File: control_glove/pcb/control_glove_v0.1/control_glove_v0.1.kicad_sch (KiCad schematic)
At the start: 14 parts, among them P1 Power_Pins, SW1 SW_Push, SW2 SW_Push, U1 UART-RF433

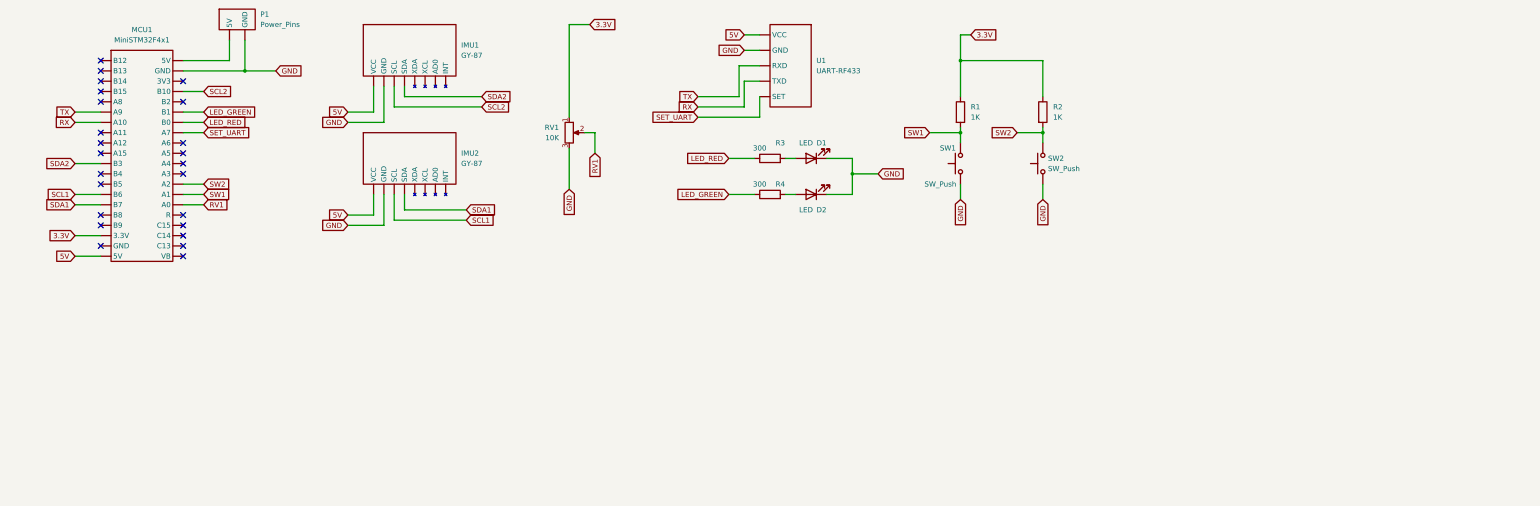
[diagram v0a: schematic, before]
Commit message: update: Complete list and connect all components
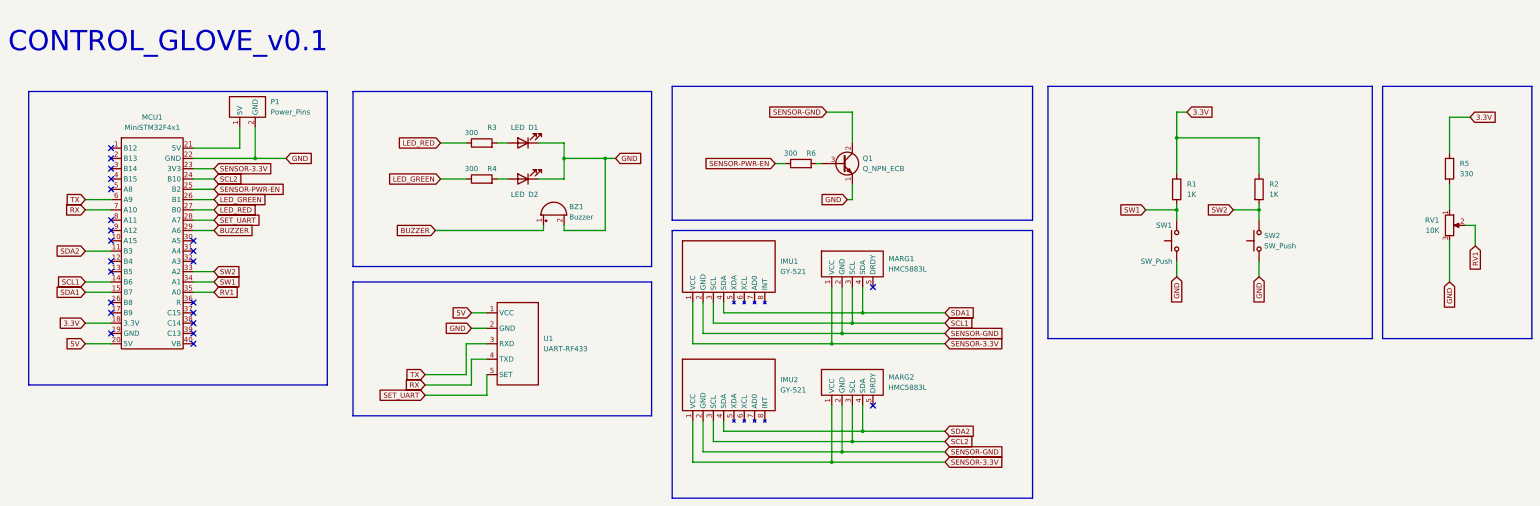
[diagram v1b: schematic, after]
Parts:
- removed IMU1, IMU2: GY-87, symbol hieu_lib:GY-87
- added BZ1: Buzzer, Buzzer_Beeper:Buzzer_12x9.5RM7.6, symbol Device:Buzzer
- added IMU1, IMU2: GY-521, Connector_PinHeader_2.54mm:PinHeader_1x08_P2.54mm_Vertical, symbol hieu_lib:GY-521
- added MARG1, MARG2: HMC5883L, Connector_PinHeader_2.54mm:PinHeader_1x05_P2.54mm_Vertical, symbol hieu_lib:HMC5883L
- added Q1: Q_NPN_ECB, Package_TO_SOT_THT:TO-92_Inline, symbol Device:Q_NPN_ECB
- added R5: 330, Resistor_THT:R_Axial_DIN0207_L6.3mm_D2.5mm_P7.62mm_Horizontal, symbol Device:R
- added R6: 300, Resistor_THT:R_Axial_DIN0207_L6.3mm_D2.5mm_P7.62mm_Horizontal, symbol Device:R
- D1, D2: footprint (none) -> LED_THT:LED_D3.0mm
- MCU1: footprint (none) -> Connector_PinHeader_2.54mm:PinHeader_2x20_P2.54mm_Vertical
- P1, SW1, SW2: footprint (none) -> TerminalBlock:TerminalBlock_Altech_AK300-2_P5.00mm
- R1, R2, R3, R4: footprint (none) -> Resistor_THT:R_Axial_DIN0207_L6.3mm_D2.5mm_P7.62mm_Horizontal
- RV1: footprint (none) -> TerminalBlock:TerminalBlock_Altech_AK300-3_P5.00mm
- U1: footprint (none) -> Connector_PinHeader_2.54mm:PinHeader_1x05_P2.54mm_Vertical
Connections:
- net 3.3V: now also MCU1.18 (3.3V), R5.1; no longer MCU1. (VB), RV1.1
- net 5V: now also MCU1.20 (5V), U1.1 (VCC); no longer MCU1. (VB), U1. (VCC)
- net GND: now also MCU1.22 (GND), P1.2 (GND), U1.2 (GND), BZ1.2 (+), Q1.1 (E); no longer MCU1. (VB), P1. (GND), U1. (VCC)
- net LED_GREEN: now also MCU1.26 (B1); no longer MCU1. (VB)
- net LED_RED: now also MCU1.27 (B0); no longer MCU1. (VB)
- net RV1: now also MCU1.35 (A0); no longer MCU1. (VB)
- net RX: now also MCU1.7 (A10), U1.4 (TXD); no longer MCU1. (VB), U1. (VCC)
- net SCL1: now also MCU1.14 (B6), IMU1.3 (SCL), MARG1.3 (SCL); no longer MCU1. (VB)
- net SCL2: now also MCU1.24 (B10), IMU2.3 (SCL), MARG2.3 (SCL); no longer MCU1. (VB)
- net SDA1: now also MCU1.15 (B7), IMU1.4 (SDA), MARG1.4 (SDA); no longer MCU1. (VB)
- net SDA2: now also MCU1.11 (B3), IMU2.4 (SDA), MARG2.4 (SDA); no longer MCU1. (VB)
- net SET_UART: now also MCU1.28 (A7), U1.5 (SET); no longer MCU1. (VB), U1. (VCC)
- net SW1: now also MCU1.34 (A1); no longer MCU1. (VB)
- net SW2: now also MCU1.33 (A2); no longer MCU1. (VB)
- net TX: now also MCU1.6 (A9), U1.3 (RXD); no longer MCU1. (VB), U1. (VCC)
- new net: R5.2, RV1.1
- new net: Q1.3 (B), R6.2
- new net: MCU1.21 (5V), P1.1 (5V)
- new net BUZZER: BZ1.1 (-), MCU1.29 (A6)
- new net SENSOR-3.3V: IMU1.1 (VCC), IMU2.1 (VCC), MARG1.1 (VCC), MARG2.1 (VCC), MCU1.23 (3V3)
- new net SENSOR-GND: IMU1.2 (GND), IMU2.2 (GND), MARG1.2 (GND), MARG2.2 (GND), Q1.2 (C)
- new net SENSOR-PWR-EN: MCU1.25 (B2), R6.1
- no-connect marks 24 -> 23
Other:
- note added: "CONTROL_GLOVE_v0.1"
- moved on the sheet: D1, D2, R1, R2, R3, R4, RV1, SW1, SW2
